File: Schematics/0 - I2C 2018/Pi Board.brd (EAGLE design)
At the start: 55 x 72 mm, 12 parts, among them J1 RASPBERRYPI-40-PIN-GPIO, U1 P82B715TD, X1 RJ45-8X, X2 RJ45-8X, X3 RJ45-8X, X4 RJ45-8X, X5 MKDSN1,5/2-5,08

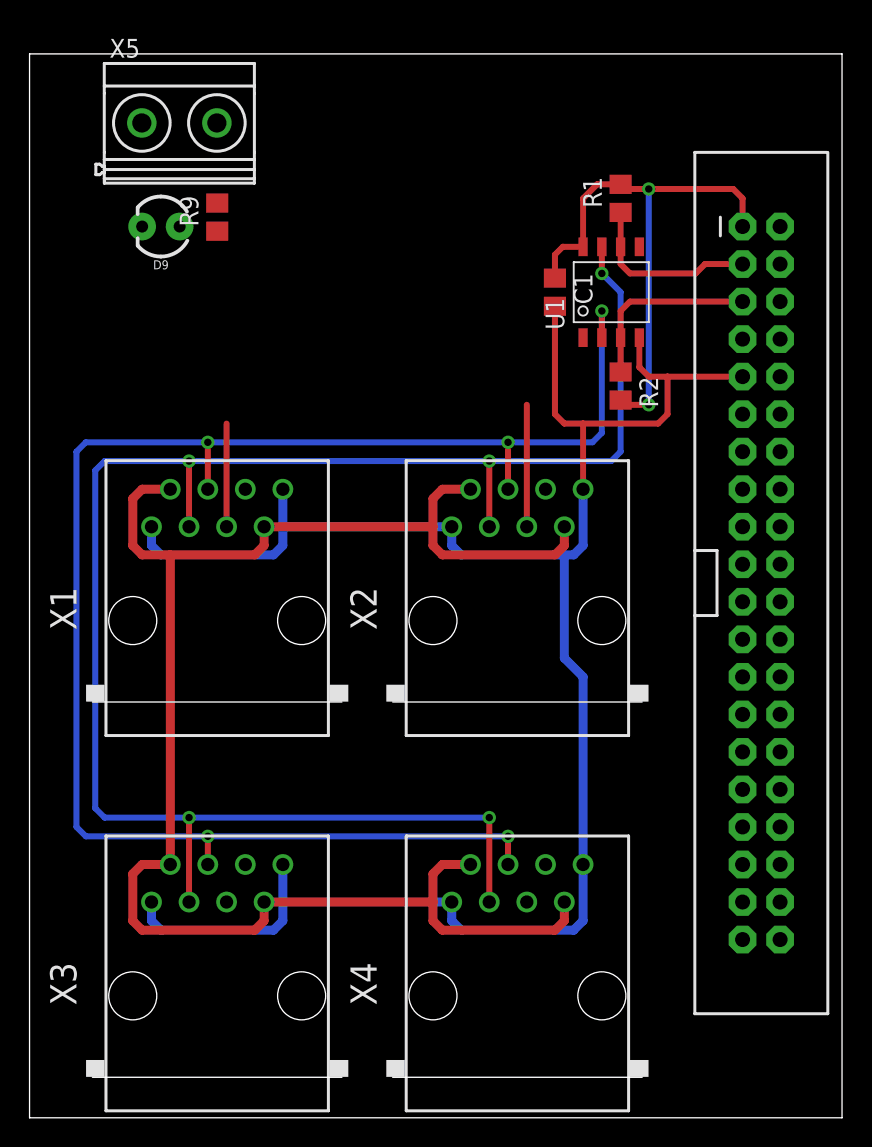
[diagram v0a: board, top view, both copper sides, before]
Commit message: Finalisation interface PI
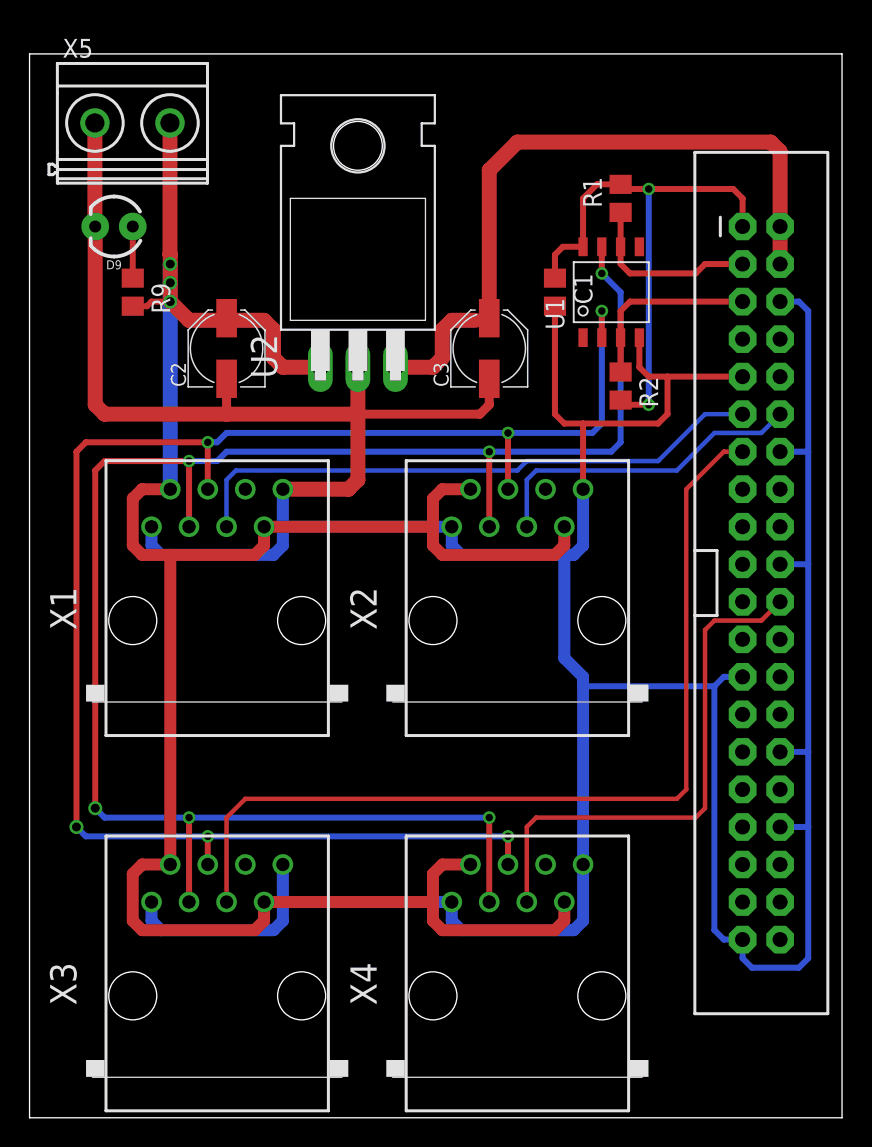
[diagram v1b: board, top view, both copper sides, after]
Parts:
- added C2, C3: (no value), resistor:PANASONIC_C
- added U2: 7805T, linear:TO220H
- moved R9 7.65 mm to (6.99, 55.9), turned to 270 degrees
- moved D9 3.18 mm to (5.71, 60.3)
- moved X5 3.17 mm to (6.99, 67.3)
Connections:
- removed net +12V: R9.2, X5.2
- removed net 5V: J1.2, J1.4
- removed net EXT_INT: X1.5, X2.5, X3.5, X4.5
- new net +5V: C3.+, J1.2, J1.4, U2.3
- new net INT_1: J1.11, X1.5
- new net INT_2: J1.12, X2.5
- new net INT_3: J1.13, X3.5
- new net INT_4: J1.22, X4.5
- net +12VBUS: now also C2.+, R9.2, U2.1, X5.2
- net DGND: now also C2.-, C3.-, U2.2
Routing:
- net DGND: track 134.0 -> 287.0 mm
- net INT_3: track 0.00 -> 62.8 mm
- net +5V: track 0.00 -> 47.2 mm
- net +12VBUS: track 110.5 -> 154.4 mm, vias 0 -> 3
- net INT_1: track 0.00 -> 39.9 mm
- net INT_4: track 0.00 -> 35.6 mm
- net INT_2: track 0.00 -> 22.2 mm
- net EXT_INT: track 15.2 -> 0.00 mm
- net N$15: track 0.00 -> 3.50 mm
- net LDA: track 120.6 -> 120.9 mm, vias 5 -> 6
- net LCL: track 111.2 -> 111.4 mm, vias 5 -> 6
